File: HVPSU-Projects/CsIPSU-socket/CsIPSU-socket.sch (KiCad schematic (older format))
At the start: 8 parts, among them J1 UFL-CONN, P1 CONN_01X10, U1 R11265U-PMT-socket

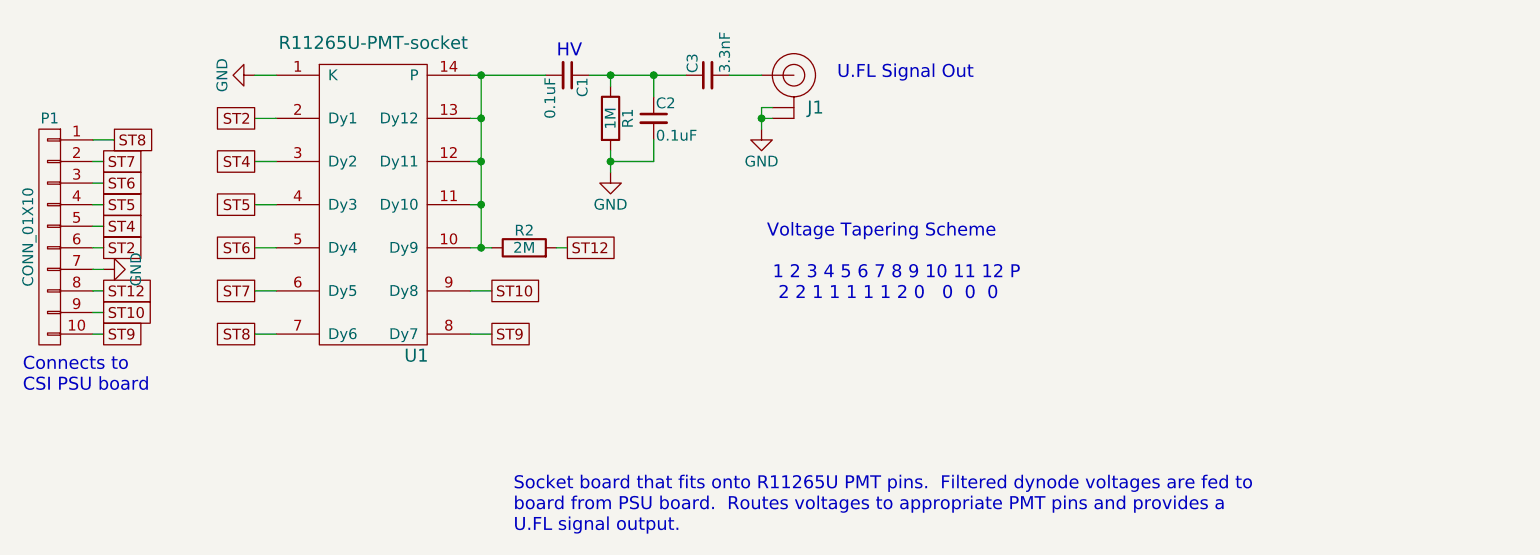
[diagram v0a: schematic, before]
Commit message: latest
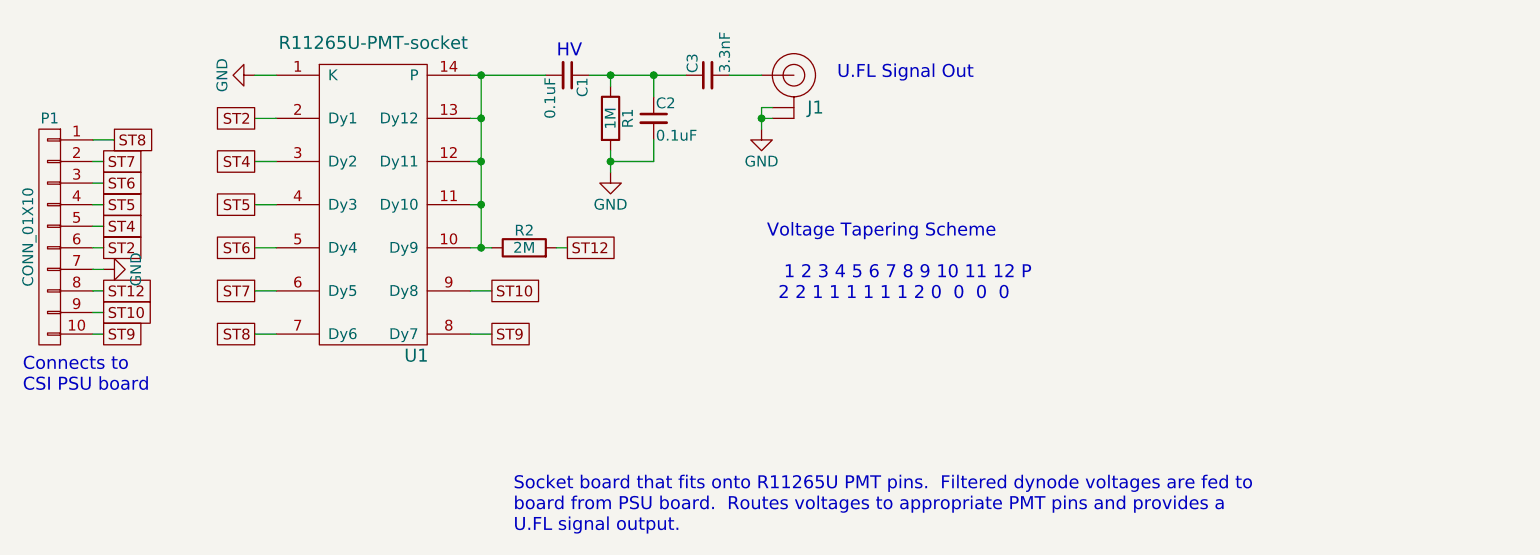
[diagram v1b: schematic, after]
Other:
- note added: "Voltage Tapering Scheme\n\n 1 2 3 4 5 6 7 8 9 10 11 12 P\n 2 2 1 1 1 1 1 1 2 0 0 0 0"
- note removed: "Voltage Tapering Scheme\n\n 1 2 3 4 5 6 7 8 9 10 11 12 P\n 2 2 1 1 1 1 1 2 0 0 0 0"
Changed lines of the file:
@@
 Socket board that fits onto R11265U PMT pins.  Filtered dynode voltages are fed to \nboard from PSU board.  Routes voltages to appropriate PMT pins and provides a \nU.FL signal output.
 Text Notes 8200 5775 0    60   ~ 0
-Voltage Tapering Scheme\n\n 1 2 3 4 5 6 7 8 9 10 11 12 P\n  2 2 1 1 1 1 1 2 0   0  0  0
+Voltage Tapering Scheme\n\n   1 2 3 4 5 6 7 8 9 10 11 12 P\n  2 2 1 1 1 1 1 1 2 0  0  0  0
 $EndSCHEMATC
